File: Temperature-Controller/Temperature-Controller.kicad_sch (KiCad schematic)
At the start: 20 parts, among them J1 RGB LED Terminal, J2 DS18B20 Terminal, J3 SSR_25DA Terminal, J4 Power Input Terminal, J5 SCT-013-020 Current Sensor Te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, J6 Red LED Power Indecator

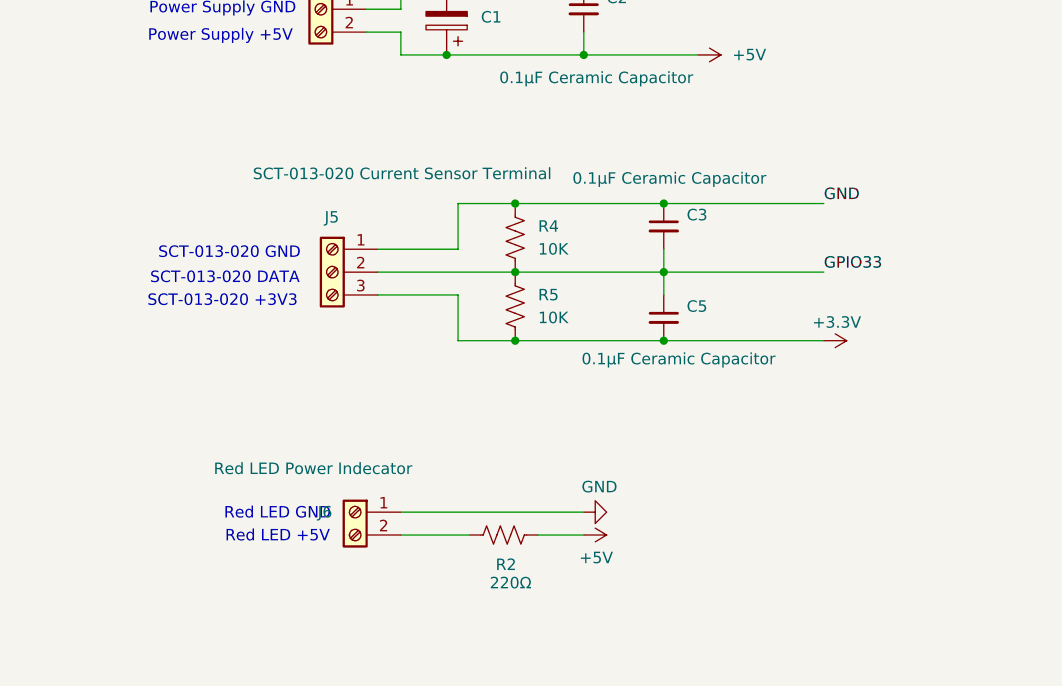
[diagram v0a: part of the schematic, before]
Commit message: Ready for creating the Gerber files
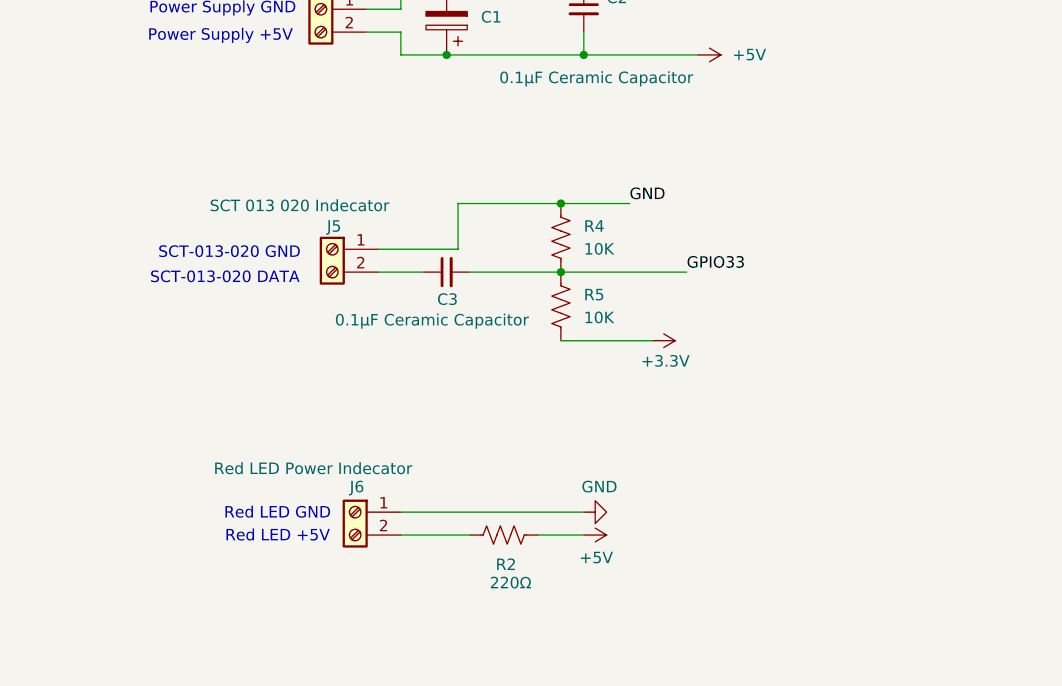
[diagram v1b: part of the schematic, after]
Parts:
- removed C5: 0.1µF Ceramic Capacitor, ESP32_Custom_Footprints:C_Disc_D3.0mm_W1.6mm_P2.50mm, symbol ESP32-Custom-Symbols:C_Small
- removed J5: SCT-013-020 Current Sensor Terminal, ESP32_Custom_Footprints:TerminalBlock_bornier-3_P5.08mm, symbol ESP32-Custom-Symbols:Screw_Terminal_01x03
- added J5: SCT 013 020 Indecator, ESP32_Custom_Footprints:TerminalBlock_bornier-2_P5.08mm, symbol ESP32-Custom-Symbols:Screw_Terminal_01x02
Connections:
- net GND: now also J5.1 (Pin_1); no longer C3.1
- new net: C3.1, J5.2 (Pin_2)
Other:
- note removed: "SCT-013-020 +3V3"
- moved on the sheet: C3, R4, R5
